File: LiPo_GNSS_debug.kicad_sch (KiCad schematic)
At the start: 7 parts

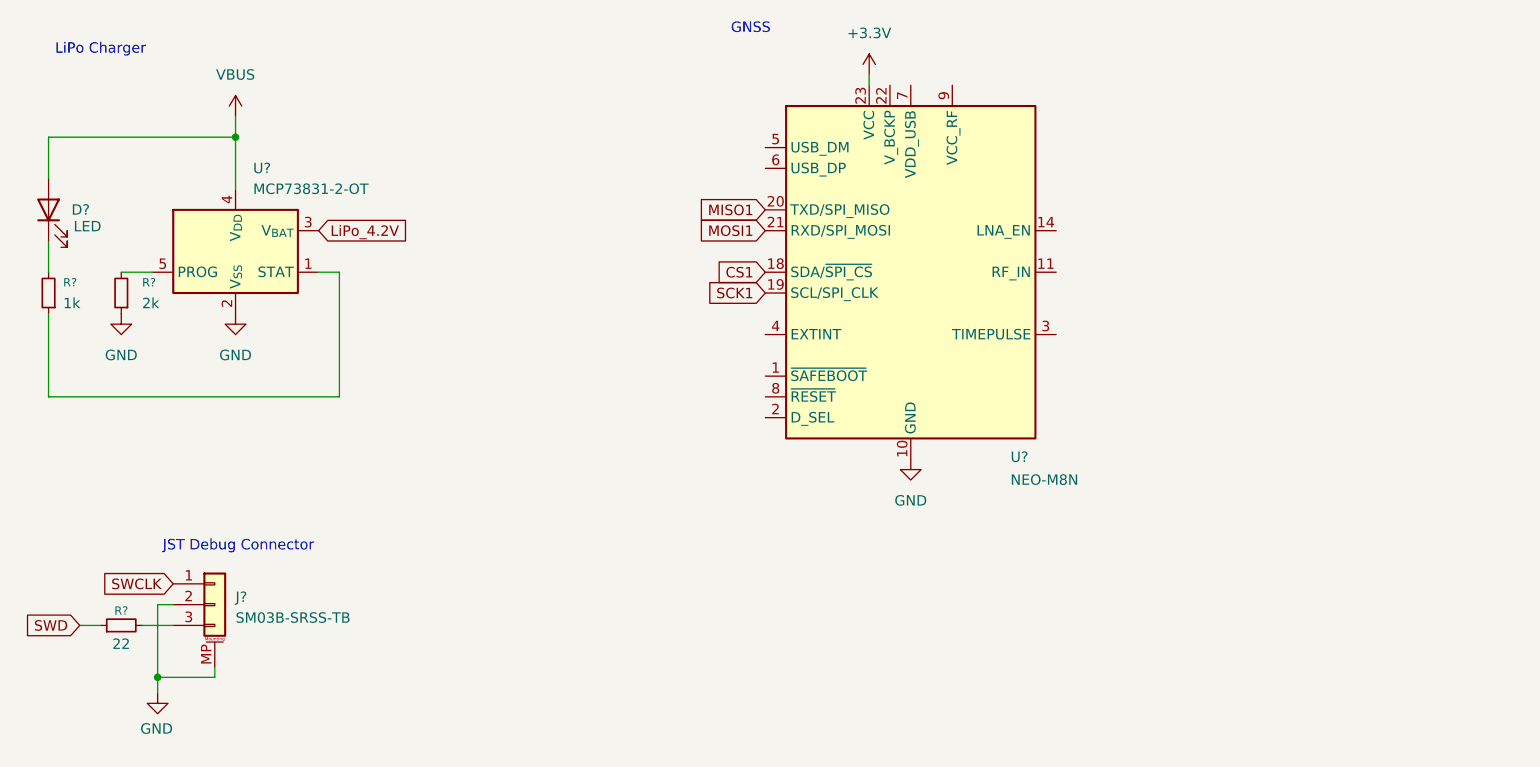
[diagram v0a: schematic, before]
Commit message: gnss_lipo_debug
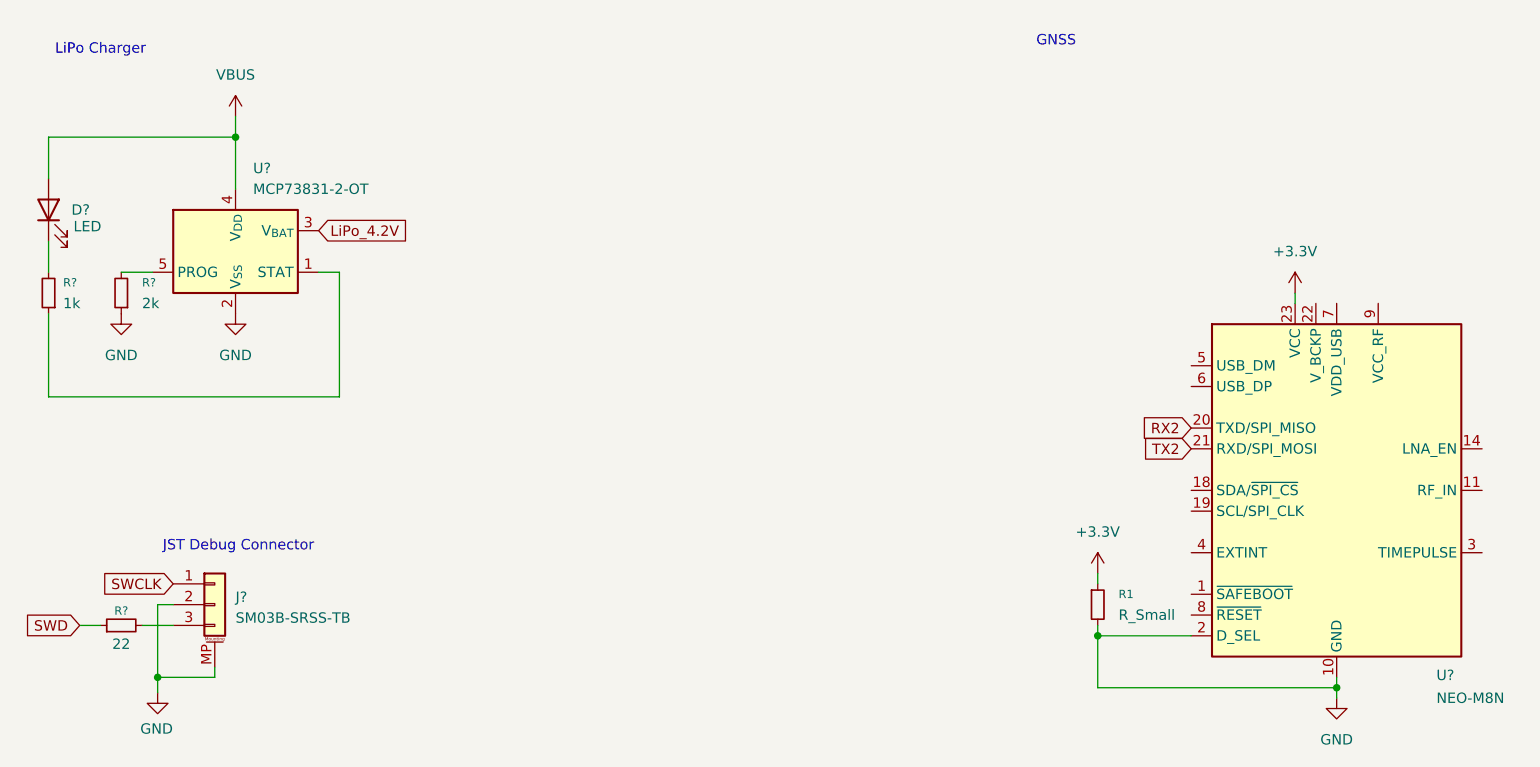
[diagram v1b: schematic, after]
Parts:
- added R1: R_Small, symbol Device:R_Small
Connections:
- net +3.3V: now also R1.1
- net GND: now also U?.2 (D_SEL), R1.2
- net CS1: no longer names the net of U?.18 (SDA/~{SPI_CS})
- net MISO1 renamed RX2
- net MOSI1 renamed TX2
- net SCK1: no longer names the net of U?.19 (SCL/SPI_CLK)
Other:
- moved on the sheet: U?
